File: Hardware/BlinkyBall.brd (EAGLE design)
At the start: 3 parts, among them IC3 TINY13-20SSU

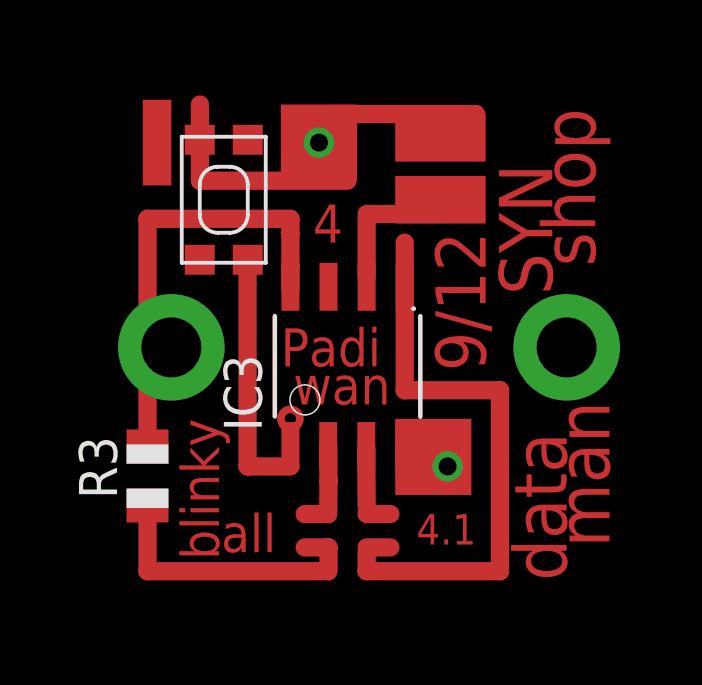
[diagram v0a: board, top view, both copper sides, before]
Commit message: Adjust for LED
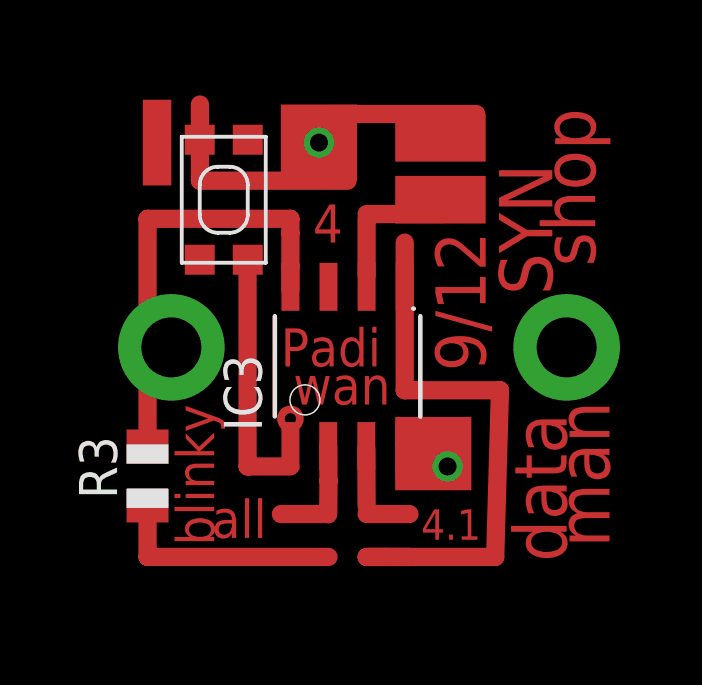
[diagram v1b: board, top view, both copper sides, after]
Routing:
- net S$13: track 1.59 -> 0.00 mm
- net S$11: track 19.2 -> 17.9 mm
- net S$8: track 0.63 -> 1.43 mm
- net S$6: track 0.79 -> 1.43 mm
- net S$2: track 5.71 -> 6.35 mm
- net N$28: track 8.24 -> 7.73 mm
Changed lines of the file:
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@@
 <text x="14.605" y="9.2075" size="1.6764" layer="1" rot="R90">9/12</text>
 <rectangle x1="7.77875" y1="15.5575" x2="10.31875" y2="18.0975" layer="1"/>
-<rectangle x1="11.58875" y1="5.08" x2="14.12875" y2="7.62" layer="1"/>
+<rectangle x1="11.58875" y1="5.23875" x2="14.12875" y2="7.6835" layer="1"/>
 <rectangle x1="11.58875" y1="16.1925" x2="14.605" y2="17.78" layer="1"/>
 <rectangle x1="11.58875" y1="14.12875" x2="14.605" y2="15.71625" layer="1"/>
 <text x="16.8275" y="11.7475" size="1.778" layer="1" rot="R90">SYN</text>
 <text x="18.7325" y="3.33375" size="1.778" layer="1" rot="R90">man</text>
-<text x="4.445" y="7.62" size="1.27" layer="1" rot="R270">blinky</text>
-<text x="7.62" y="4.445" size="1.27" layer="1" rot="R180">all</text>
-<text x="14.2875" y="4.445" size="1.016" layer="1" rot="R180">4.1</text>
+<text x="4.28625" y="8.09625" size="1.27" layer="1" rot="R270">blinky</text>
+<text x="7.3025" y="4.92125" size="1.27" layer="1" rot="R180">all</text>
+<text x="14.44625" y="4.60375" size="1.016" layer="1" rot="R180">4.1</text>
 <text x="18.25625" y="12.7" size="1.778" layer="1" rot="R90">shop</text>
-<text x="17.30375" y="2.2225" size="1.778" layer="1" rot="R90">data</text>
+<text x="17.30375" y="2.8575" size="1.778" layer="1" rot="R90">data</text>
 <text x="11.1125" y="10.63625" size="1.27" layer="1" rot="R180">Padi</text>
 <text x="11.43" y="9.36625" size="1.27" layer="1" rot="R180">wan</text>
@@
 <signal name="N$28">
 <contactref element="R3" pad="1"/>
-<wire x1="9.36625" y1="2.425" x2="9.2075" y2="2.54" width="0.4064" layer="1"/>
-<wire x1="9.2075" y1="2.54" x2="3.33375" y2="2.54" width="0.6096" layer="1"/>
-<wire x1="3.33375" y1="2.54" x2="3.33375" y2="4.715" width="0.6096" layer="1"/>
+<wire x1="9.36625" y1="3.01625" x2="3.33375" y2="3.01625" width="0.6096" layer="1"/>
+<wire x1="3.33375" y1="3.01625" x2="3.33375" y2="4.715" width="0.6096" layer="1"/>
 </signal>
 <signal name="N$30">
@@
 <wire x1="11.89625" y1="6.71225" x2="11.89625" y2="6.82625" width="0.4064" layer="1"/>
 <wire x1="11.89625" y1="6.82625" x2="11.90625" y2="6.82625" width="0.6096" layer="1"/>
-<wire x1="11.90625" y1="6.82625" x2="11.90625" y2="5.715" width="0.6096" layer="1"/>
+<wire x1="11.90625" y1="6.82625" x2="11.90625" y2="5.588" width="0.6096" layer="1"/>
 </signal>
 <signal name="N$15">
@@
 </signal>
 <signal name="S$2">
-<wire x1="10.63625" y1="4.445" x2="11.43" y2="4.445" width="0.6096" layer="1"/>
+<wire x1="10.63625" y1="4.445" x2="12.065" y2="4.445" width="0.6096" layer="1"/>
 <wire x1="9.36625" y1="17.78" x2="14.2875" y2="17.78" width="0.6096" layer="1"/>
 </signal>
@@
 <signal name="S$11">
 <wire x1="11.90625" y1="13.49375" x2="11.90625" y2="8.5725" width="0.6096" layer="1"/>
-<wire x1="15.08125" y1="8.5725" x2="15.08125" y2="2.54" width="0.6096" layer="1"/>
-<wire x1="15.08125" y1="2.54" x2="10.63625" y2="2.54" width="0.6096" layer="1"/>
+<wire x1="15.08125" y1="8.5725" x2="14.9225" y2="3.01625" width="0.6096" layer="1"/>
+<wire x1="14.9225" y1="3.01625" x2="11.27125" y2="3.01625" width="0.6096" layer="1"/>
 <wire x1="11.90625" y1="8.5725" x2="15.08125" y2="8.5725" width="0.6096" layer="1"/>
-<wire x1="10.63625" y1="2.54" x2="10.63625" y2="3.175" width="0.6096" layer="1"/>
+<wire x1="11.27125" y1="3.01625" x2="10.63625" y2="3.01625" width="0.6096" layer="1"/>
 </signal>
 <signal name="S$12">
@@
 </signal>
 <signal name="S$8">
-<wire x1="9.2075" y1="4.445" x2="8.5725" y2="4.445" width="0.6096" layer="1"/>
-</signal>
-<signal name="S$13">
-<wire x1="9.36625" y1="2.54" x2="9.36625" y2="3.33375" width="0.6096" layer="1"/>
-<wire x1="9.36625" y1="3.33375" x2="8.5725" y2="3.33375" width="0.6096" layer="1"/>
+<wire x1="9.2075" y1="4.445" x2="7.77875" y2="4.445" width="0.6096" layer="1"/>
 </signal>
 <signal name="S$1">
@@
 </signal>
 <signal name="S$6">
-<wire x1="10.63625" y1="3.33375" x2="11.43" y2="3.33375" width="0.6096" layer="1"/>
+<wire x1="10.63625" y1="3.01625" x2="12.065" y2="3.01625" width="0.6096" layer="1"/>
 </signal>
 <signal name="S$9">
